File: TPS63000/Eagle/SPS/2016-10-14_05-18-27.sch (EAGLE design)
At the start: 11 parts, among them U1 TPS63000DRCR

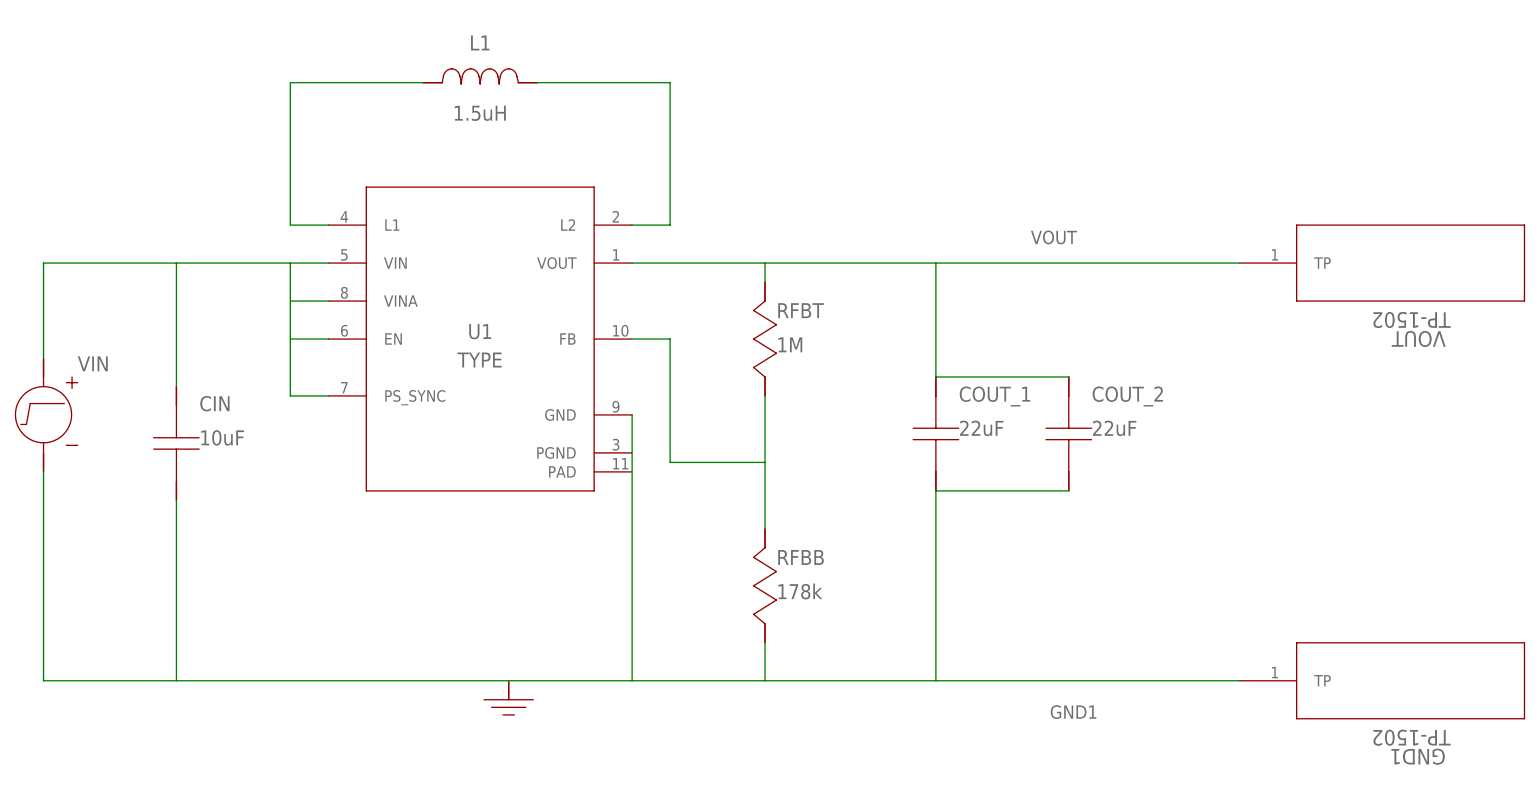
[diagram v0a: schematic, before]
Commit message: finished the schematic and board designs
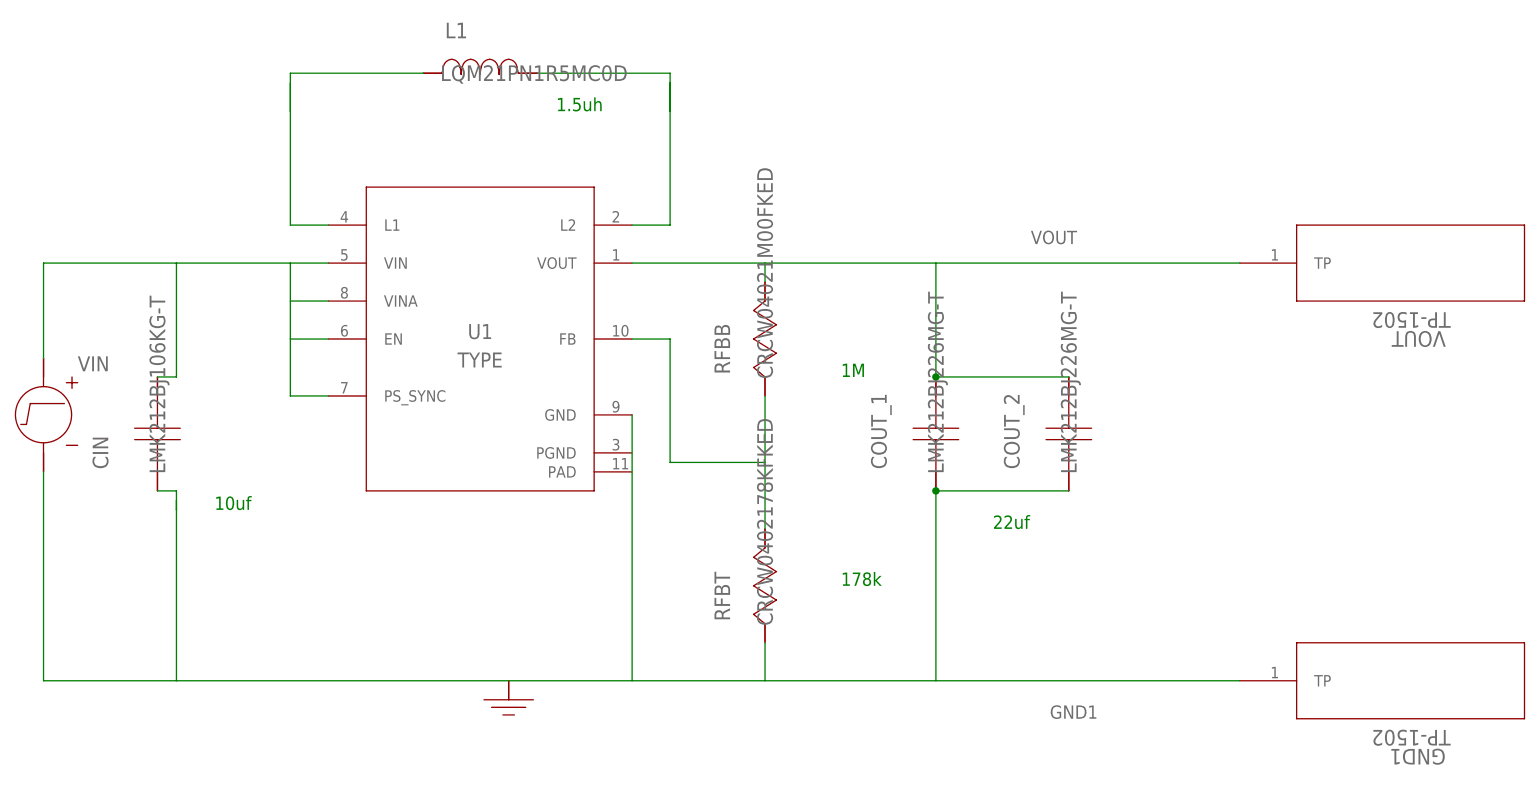
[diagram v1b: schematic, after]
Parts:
- CIN: value 10uF -> LMK212BJ106KG-T; device AcceleratedDesigns_Lib:LMK212BJ106KG-TLMK212BJ106KG-T -> sps:LMK212BJ106KG-T
- COUT_1, COUT_2: value 22uF -> LMK212BJ226MG-T; device AcceleratedDesigns_Lib:LMK212BJ226MG-TLMK212BJ226MG-T -> sps:LMK212BJ226MG-T
- L1: value 1.5uH -> LQM21PN1R5MC0D; device AcceleratedDesigns_Lib:LQM21PN1R5MC0DLQM21PN1R5MC0D -> sps:LQM21PN1R5MC0D
- RFBB: value 178k -> CRCW04021M00FKED; device AcceleratedDesigns_Lib:CRCW0402178KFKEDCRCW0402178KFKED -> sps:CRCW04021M00FKED
- RFBT: value 1M -> CRCW0402178KFKED; device AcceleratedDesigns_Lib:CRCW04021M00FKEDCRCW04021M00FKED -> sps:CRCW0402178KFKED
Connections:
- new net N$3: U1.EN@6
- net 1: now also CIN.1; no longer CIN.1@1, U1.EN@6
- net 2: now also L1.1; no longer L1.1@1
- net 3: now also RFBB.2, RFBT.1; no longer RFBB.1@1, RFBT.2@2
- net 4: now also L1.2; no longer L1.2@2
- net GND1: now also CIN.2, COUT_1.2, COUT_2.2; no longer CIN.2@2, COUT_1.2@2, COUT_2.2@2
- net N$1: now also RFBB.1; no longer RFBT.1@1
- net N$2: now also RFBT.2; no longer RFBB.2@2
- net VOUT: now also COUT_1.1, COUT_2.1; no longer COUT_1.1@1, COUT_2.1@1
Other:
- note added: "1.5uh"
- note added: "10uf"
- note added: "178k"
- note added: "1M"
- note added: "22uf"
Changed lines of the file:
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@@
 </classes>
 <parts>
-<part name="CIN" library="AcceleratedDesigns_Lib" deviceset="LMK212BJ106KG-T" device="LMK212BJ106KG-T" value="10uF"/>
-<part name="COUT_1" library="AcceleratedDesigns_Lib" deviceset="LMK212BJ226MG-T" device="LMK212BJ226MG-T" value="22uF"/>
 <part name="GND" library="AcceleratedDesigns_Lib" deviceset="WB_GND" device="WB_GND" value="WB_GND"/>
-<part name="L1" library="AcceleratedDesigns_Lib" deviceset="LQM21PN1R5MC0D" device="LQM21PN1R5MC0D" value="1.5uH"/>
-<part name="RFBB" library="AcceleratedDesigns_Lib" deviceset="CRCW0402178KFKED" device="CRCW0402178KFKED" value="178k"/>
-<part name="RFBT" library="AcceleratedDesigns_Lib" deviceset="CRCW04021M00FKED" device="CRCW04021M00FKED" value="1M"/>
 <part name="U1" library="AcceleratedDesigns_Lib" deviceset="TPS63000DRCR" device="TPS63000DRCR" value="TPS63000DRCR"/>
 <part name="VIN" library="AcceleratedDesigns_Lib" deviceset="WB_STARTUP_VOLTAGE_SOURCE" device="WB_STARTUP_VOLTAGE_SOURCE" value="WB_STARTUP_VOLTAGE_SOURCE"/>
-<part name="COUT_2" library="AcceleratedDesigns_Lib" deviceset="LMK212BJ226MG-T" device="LMK212BJ226MG-T" value="22uF"/>
 <part name="VOUT" library="sps" deviceset="TP-1502" device=""/>
 <part name="GND1" library="sps" deviceset="TP-1502" device=""/>
+<part name="RFBB" library="sps" deviceset="CRCW04021M00FKED" device=""/>
+<part name="RFBT" library="sps" deviceset="CRCW0402178KFKED" device=""/>
+<part name="CIN" library="sps" deviceset="LMK212BJ106KG-T" device=""/>
+<part name="COUT_1" library="sps" deviceset="LMK212BJ226MG-T" device=""/>
+<part name="COUT_2" library="sps" deviceset="LMK212BJ226MG-T" device=""/>
+<part name="L1" library="sps" deviceset="LQM21PN1R5MC0D" device=""/>
 </parts>
 <sheets>
 <sheet>
 <plain>
+<text x="53.34" y="53.34" size="1.778" layer="91">10uf</text>
+<text x="157.48" y="50.8" size="1.778" layer="91">22uf</text>
+<text x="99.06" y="106.68" size="1.778" layer="91">1.5uh</text>
+<text x="137.16" y="71.12" size="1.778" layer="91">1M</text>
+<text x="137.16" y="43.18" size="1.778" layer="91">178k</text>
 </plain>
 <instances>
-<instance part="CIN" gate="1" x="48.26" y="62.23" smashed="yes" rot="R90">
-<attribute name="NAME" x="51.308" y="66.548" size="2" layer="95"/>
-<attribute name="VALUE" x="51.308" y="61.976" size="2" layer="96"/>
-</instance>
-<instance part="COUT_1" gate="1" x="149.86" y="63.5" smashed="yes" rot="R90">
-<attribute name="NAME" x="152.908" y="67.818" size="2" layer="95"/>
-<attribute name="VALUE" x="152.908" y="63.246" size="2" layer="96"/>
-</instance>
 <instance part="GND" gate="1" x="92.71" y="27.94" smashed="yes">
 <attribute name="NAME" x="92.71" y="33.528" size="2" layer="95" align="bottom-center" display="off"/>
-</instance>
-<instance part="L1" gate="1" x="88.9" y="110.49" smashed="yes">
-<attribute name="NAME" x="88.9" y="114.808" size="2" layer="95" align="bottom-center"/>
-<attribute name="VALUE" x="88.9" y="105.41" size="2" layer="96" align="bottom-center"/>
-</instance>
-<instance part="RFBB" gate="1" x="127" y="43.18" smashed="yes" rot="R90">
-<attribute name="NAME" x="128.524" y="45.974" size="2" layer="95"/>
-<attribute name="VALUE" x="128.524" y="41.402" size="2" layer="96"/>
-</instance>
-<instance part="RFBT" gate="1" x="127" y="76.2" smashed="yes" rot="R90">
-<attribute name="NAME" x="128.524" y="78.994" size="2" layer="95"/>
-<attribute name="VALUE" x="128.524" y="74.422" size="2" layer="96"/>
 </instance>
 <instance part="U1" gate="1" x="88.9" y="76.2" smashed="yes">
@@
 <attribute name="NAME" x="35.052" y="71.882" size="2" layer="95"/>
 </instance>
-<instance part="COUT_2" gate="1" x="167.64" y="63.5" smashed="yes" rot="R90">
-<attribute name="NAME" x="170.688" y="67.818" size="2" layer="95"/>
-<attribute name="VALUE" x="170.688" y="63.246" size="2" layer="96"/>
-</instance>
 <instance part="VOUT" gate="A" x="190.5" y="86.36" rot="R180"/>
 <instance part="GND1" gate="A" x="190.5" y="30.48" rot="R180"/>
+<instance part="RFBB" gate="A" x="127" y="76.2" rot="R90"/>
+<instance part="RFBT" gate="A" x="127" y="43.18" rot="R90"/>
+<instance part="CIN" gate="A" x="45.72" y="63.5" rot="R90"/>
+<instance part="COUT_1" gate="A" x="149.86" y="63.5" rot="R90"/>
+<instance part="COUT_2" gate="A" x="167.64" y="63.5" rot="R90"/>
+<instance part="L1" gate="A" x="88.9" y="111.76"/>
 </instances>
 <busses>
@@
 <net name="1" class="0">
 <segment>
-<pinref part="CIN" gate="1" pin="1@1"/>
+<wire x1="63.5" y1="68.58" x2="63.5" y2="86.36" width="0" layer="91"/>
+<pinref part="U1" gate="1" pin="PS_SYNC@7"/>
+<wire x1="68.58" y1="68.58" x2="63.5" y2="68.58" width="0" layer="91"/>
+</segment>
+<segment>
+<wire x1="48.26" y1="71.12" x2="48.26" y2="86.36" width="0" layer="91"/>
+<pinref part="CIN" gate="A" pin="1"/>
+<wire x1="45.72" y1="71.12" x2="48.26" y2="71.12" width="0.1524" layer="91"/>
+</segment>
+<segment>
+<pinref part="U1" gate="1" pin="VINA@8"/>
+<wire x1="68.58" y1="81.28" x2="63.5" y2="81.28" width="0" layer="91"/>
+</segment>
+<segment>
 <pinref part="U1" gate="1" pin="VIN@5"/>
-<pinref part="U1" gate="1" pin="EN@6"/>
-<pinref part="U1" gate="1" pin="PS_SYNC@7"/>
-<pinref part="U1" gate="1" pin="VINA@8"/>
 <pinref part="VIN" gate="1" pin="+@1"/>
-<wire x1="63.5" y1="68.58" x2="63.5" y2="86.36" width="0" layer="91"/>
-<wire x1="68.58" y1="68.58" x2="63.5" y2="68.58" width="0" layer="91"/>
-<wire x1="68.58" y1="76.2" x2="63.5" y2="76.2" width="0" layer="91"/>
-<wire x1="68.58" y1="81.28" x2="63.5" y2="81.28" width="0" layer="91"/>
-<wire x1="48.26" y1="69.85" x2="48.26" y2="86.36" width="0" layer="91"/>
 <wire x1="30.48" y1="86.36" x2="68.58" y2="86.36" width="0" layer="91"/>
 <wire x1="30.48" y1="73.66" x2="30.48" y2="86.36" width="0" layer="91"/>
@@
 </segment>
 <segment>
-<pinref part="CIN" gate="1" pin="2@2"/>
-<wire x1="48.26" y1="54.61" x2="48.26" y2="30.48" width="0" layer="91"/>
+<wire x1="48.26" y1="54.61" x2="48.26" y2="53.34" width="0" layer="91"/>
+<pinref part="CIN" gate="A" pin="2"/>
+<wire x1="48.26" y1="53.34" x2="48.26" y2="30.48" width="0" layer="91"/>
+<wire x1="45.72" y1="55.88" x2="48.26" y2="55.88" width="0.1524" layer="91"/>
+<wire x1="48.26" y1="53.34" x2="48.26" y2="55.88" width="0.1524" layer="91"/>
 </segment>
 <segment>
-<pinref part="COUT_2" gate="1" pin="2@2"/>
-<pinref part="COUT_1" gate="1" pin="2@2"/>
 <wire x1="149.86" y1="55.88" x2="167.64" y2="55.88" width="0" layer="91"/>
 <wire x1="149.86" y1="55.88" x2="149.86" y2="30.48" width="0" layer="91"/>
+<pinref part="COUT_1" gate="A" pin="2"/>
+<junction x="149.86" y="55.88"/>
+<pinref part="COUT_2" gate="A" pin="2"/>
 </segment>
 <segment>
@@
 <net name="VOUT" class="0">
 <segment>
-<pinref part="COUT_2" gate="1" pin="1@1"/>
-<pinref part="COUT_1" gate="1" pin="1@1"/>
 <wire x1="149.86" y1="71.12" x2="149.86" y2="86.36" width="0" layer="91"/>
 <wire x1="149.86" y1="71.12" x2="167.64" y2="71.12" width="0" layer="91"/>
+<pinref part="COUT_1" gate="A" pin="1"/>
+<junction x="149.86" y="71.12"/>
+<pinref part="COUT_2" gate="A" pin="1"/>
 </segment>
 <segment>
@@
 <net name="2" class="0">
 <segment>
-<pinref part="L1" gate="1" pin="1@1"/>
 <pinref part="U1" gate="1" pin="L1@4"/>
-<wire x1="63.5" y1="110.49" x2="63.5" y2="91.44" width="0" layer="91"/>
+<wire x1="63.5" y1="110.49" x2="63.5" y2="106.68" width="0" layer="91"/>
+<wire x1="63.5" y1="106.68" x2="63.5" y2="91.44" width="0" layer="91"/>
 <wire x1="68.58" y1="91.44" x2="63.5" y2="91.44" width="0" layer="91"/>
-<wire x1="81.28" y1="110.49" x2="63.5" y2="110.49" width="0" layer="91"/>
+<pinref part="L1" gate="A" pin="1"/>
+<wire x1="81.28" y1="111.76" x2="63.5" y2="111.76" width="0.1524" layer="91"/>
+<wire x1="63.5" y1="111.76" x2="63.5" y2="106.68" width="0.1524" layer="91"/>
 </segment>
 </net>
 <net name="4" class="0">
 <segment>
-<pinref part="L1" gate="1" pin="2@2"/>
 <pinref part="U1" gate="1" pin="L2@2"/>
 <wire x1="109.22" y1="91.44" x2="114.3" y2="91.44" width="0" layer="91"/>
-<wire x1="114.3" y1="110.49" x2="114.3" y2="91.44" width="0" layer="91"/>
-<wire x1="96.52" y1="110.49" x2="114.3" y2="110.49" width="0" layer="91"/>
+<wire x1="114.3" y1="110.49" x2="114.3" y2="106.68" width="0" layer="91"/>
+<wire x1="114.3" y1="106.68" x2="114.3" y2="91.44" width="0" layer="91"/>
+<pinref part="L1" gate="A" pin="2"/>
+<wire x1="96.52" y1="111.76" x2="114.3" y2="111.76" width="0.1524" layer="91"/>
+<wire x1="114.3" y1="111.76" x2="114.3" y2="106.68" width="0.1524" layer="91"/>
 </segment>
 </net>
 <net name="3" class="0">
 <segment>
-<pinref part="RFBB" gate="1" pin="1@1"/>
-<pinref part="RFBT" gate="1" pin="2@2"/>
 <pinref part="U1" gate="1" pin="FB@10"/>
 <wire x1="109.22" y1="76.2" x2="114.3" y2="76.2" width="0" layer="91"/>
@@
 <wire x1="114.3" y1="76.2" x2="114.3" y2="59.69" width="0" layer="91"/>
 <wire x1="127" y1="68.58" x2="127" y2="50.8" width="0" layer="91"/>
+<pinref part="RFBB" gate="A" pin="2"/>
+<pinref part="RFBT" gate="A" pin="1"/>
 </segment>
 </net>
 <net name="N$1" class="0">
 <segment>
-<pinref part="RFBT" gate="1" pin="1@1"/>
 <wire x1="127" y1="83.82" x2="127" y2="86.36" width="0" layer="91"/>
+<pinref part="RFBB" gate="A" pin="1"/>
 </segment>
 </net>
 <net name="N$2" class="0">
 <segment>
-<pinref part="RFBB" gate="1" pin="2@2"/>
 <wire x1="127" y1="35.56" x2="127" y2="30.48" width="0" layer="91"/>
+<pinref part="RFBT" gate="A" pin="2"/>
 </segment>
 </net>
+<net name="N$3" class="0">
+<segment>
+<pinref part="U1" gate="1" pin="EN@6"/>
+<wire x1="68.58" y1="76.2" x2="63.5" y2="76.2" width="0" layer="91"/>
+</segment>
+</net>
